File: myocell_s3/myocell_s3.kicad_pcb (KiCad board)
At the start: 4 copper layers, 100 parts, among them J1 Conn_01x08, J5 Battery Connector JC2, J7 USB_C_Receptacle_USB2.0_16P, Q3 DMG3404L, SW1 SW_Push, SW2 SW_Push, U1 MSS22D18, U2 ADS1298xPAG, U4 ESP32-S3-WROOM-2, U6 AP2112K-3.3, U7 MCP73831-2-OT, U8 AP2112K-3.3

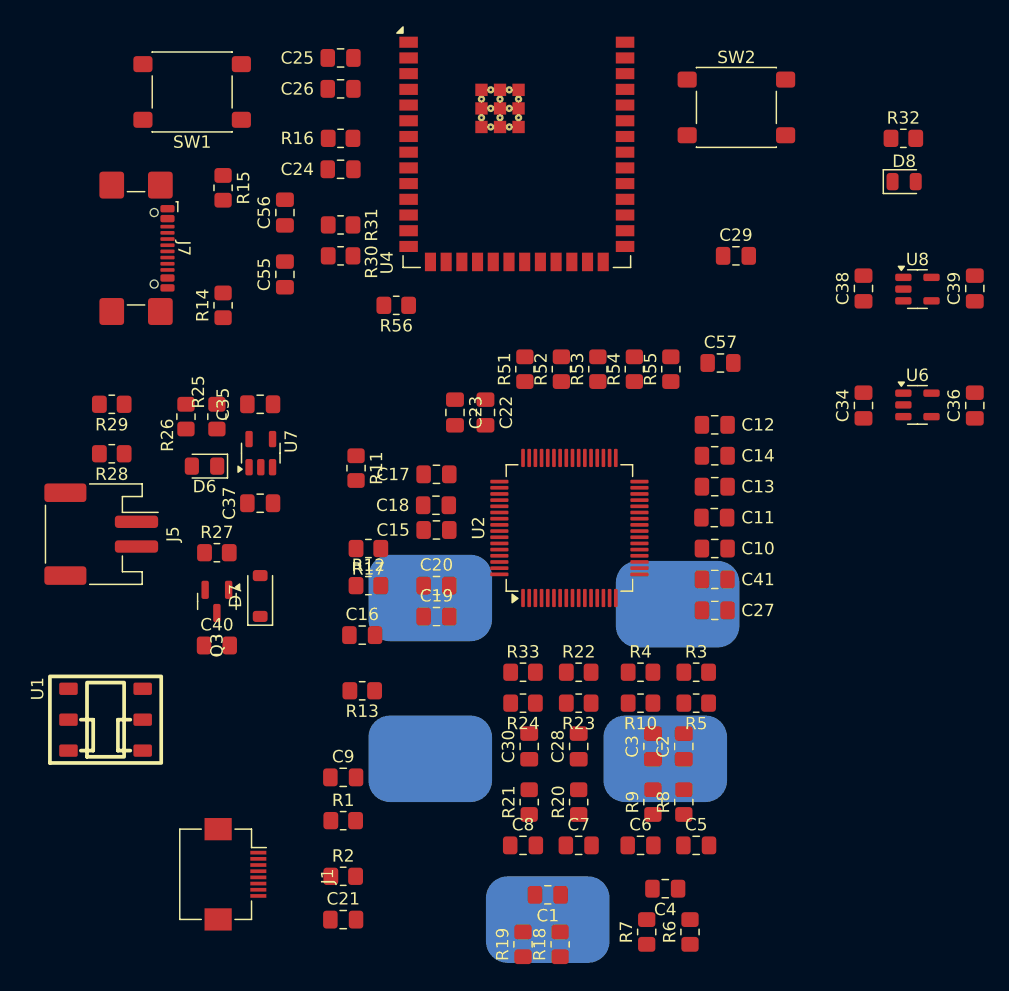
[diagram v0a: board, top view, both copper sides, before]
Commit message: working on components placement
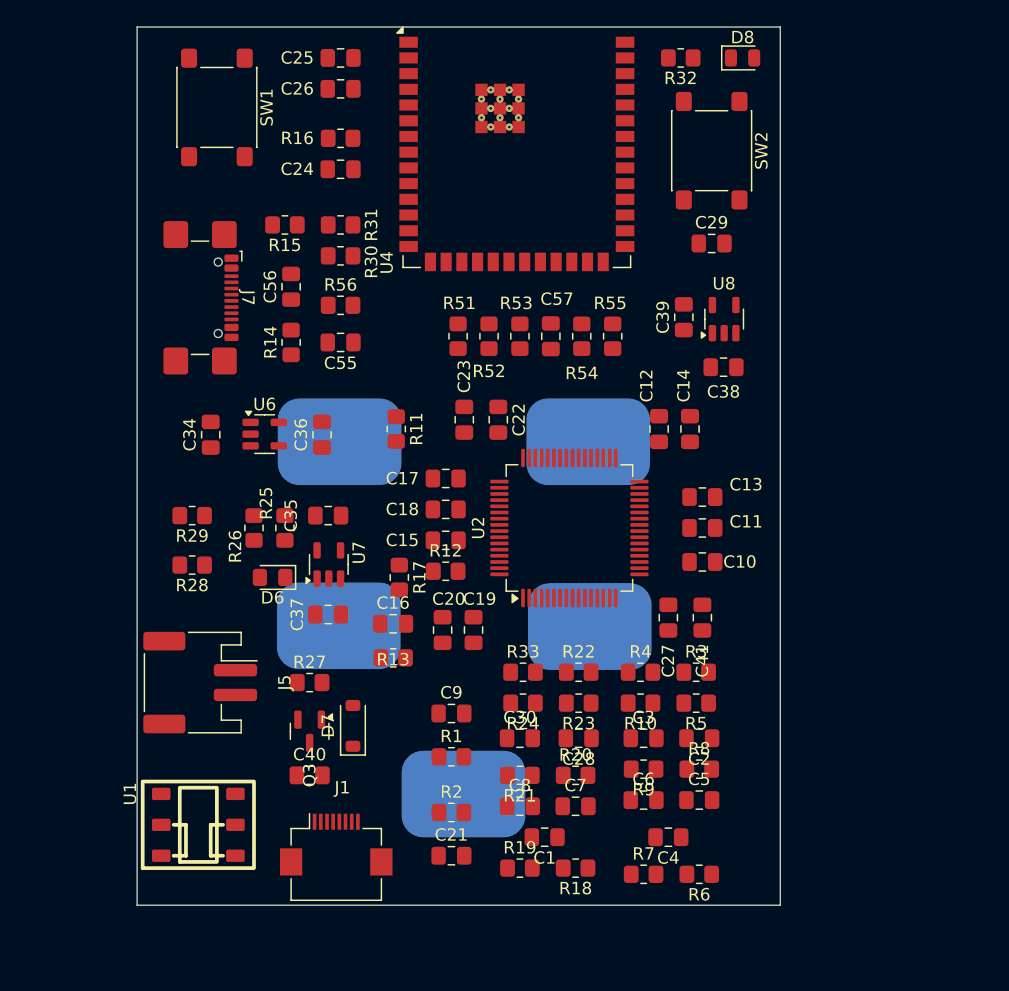
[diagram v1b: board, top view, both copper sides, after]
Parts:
- moved C34 52.8 mm to (159.5, 83.0)
- moved C36 52.8 mm to (168.5, 83.0)
- moved U6 52.8 mm to (163.9, 82.9)
- moved C39 23.6 mm to (197.8, 73.5)
- moved R32 19.1 mm to (197.5, 52.5), turned to 180 degrees
- moved D8 16.5 mm to (202.5, 52.5)
- moved U8 15.8 mm to (201.0, 73.6), turned to 90 degrees
- moved J4 15.0 mm to (190.0, 83.5)
- moved J2 14.6 mm to (169.9, 83.5)
- moved J5 14.4 mm to (158.7, 103.0)
- moved C57 13.9 mm to (187.0, 75.0), turned to 90 degrees
- moved J3 13.0 mm to (169.9, 98.4)
- moved C38 13.0 mm to (201.0, 77.5), turned to 180 degrees
- moved C40 12.9 mm to (167.5, 110.5)
- moved D7 12.9 mm to (171.0, 106.5)
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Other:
- board outline added: 52 x 71 mm
